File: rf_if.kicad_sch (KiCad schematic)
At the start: 46 parts, among them IC1 SBL-1+, Q33 2SC5171, U2 74LVC74, U3 Adafruit_Si5351, U4 74HCT244, U5 74HC4066, U6 74HC4066, U7 LM358

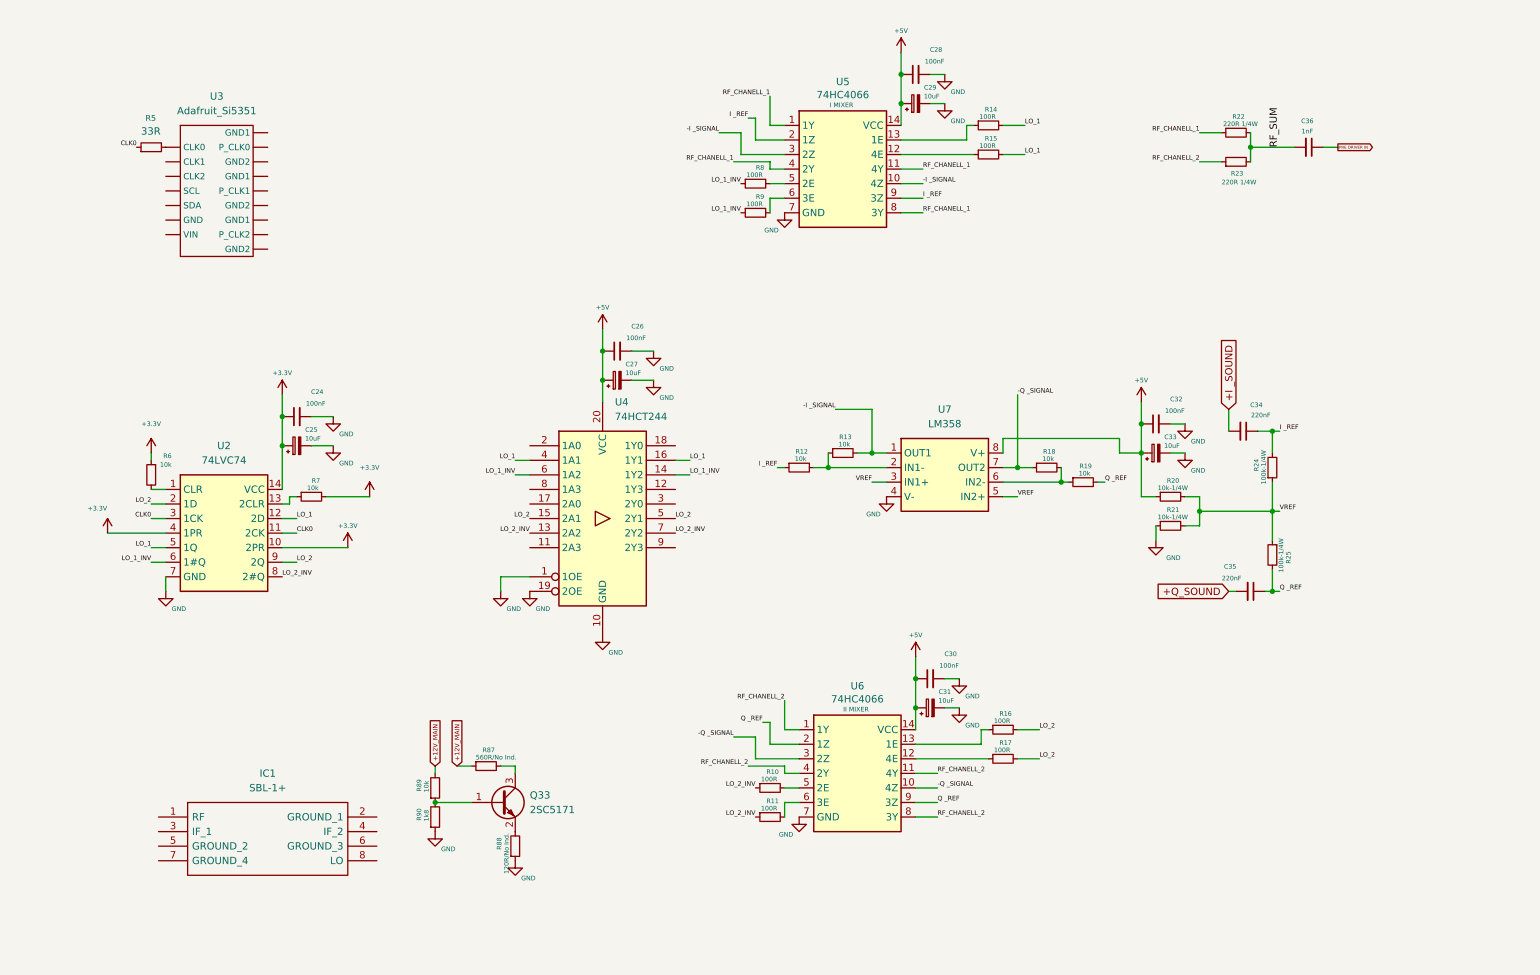
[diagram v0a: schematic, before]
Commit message: Mixer work 2
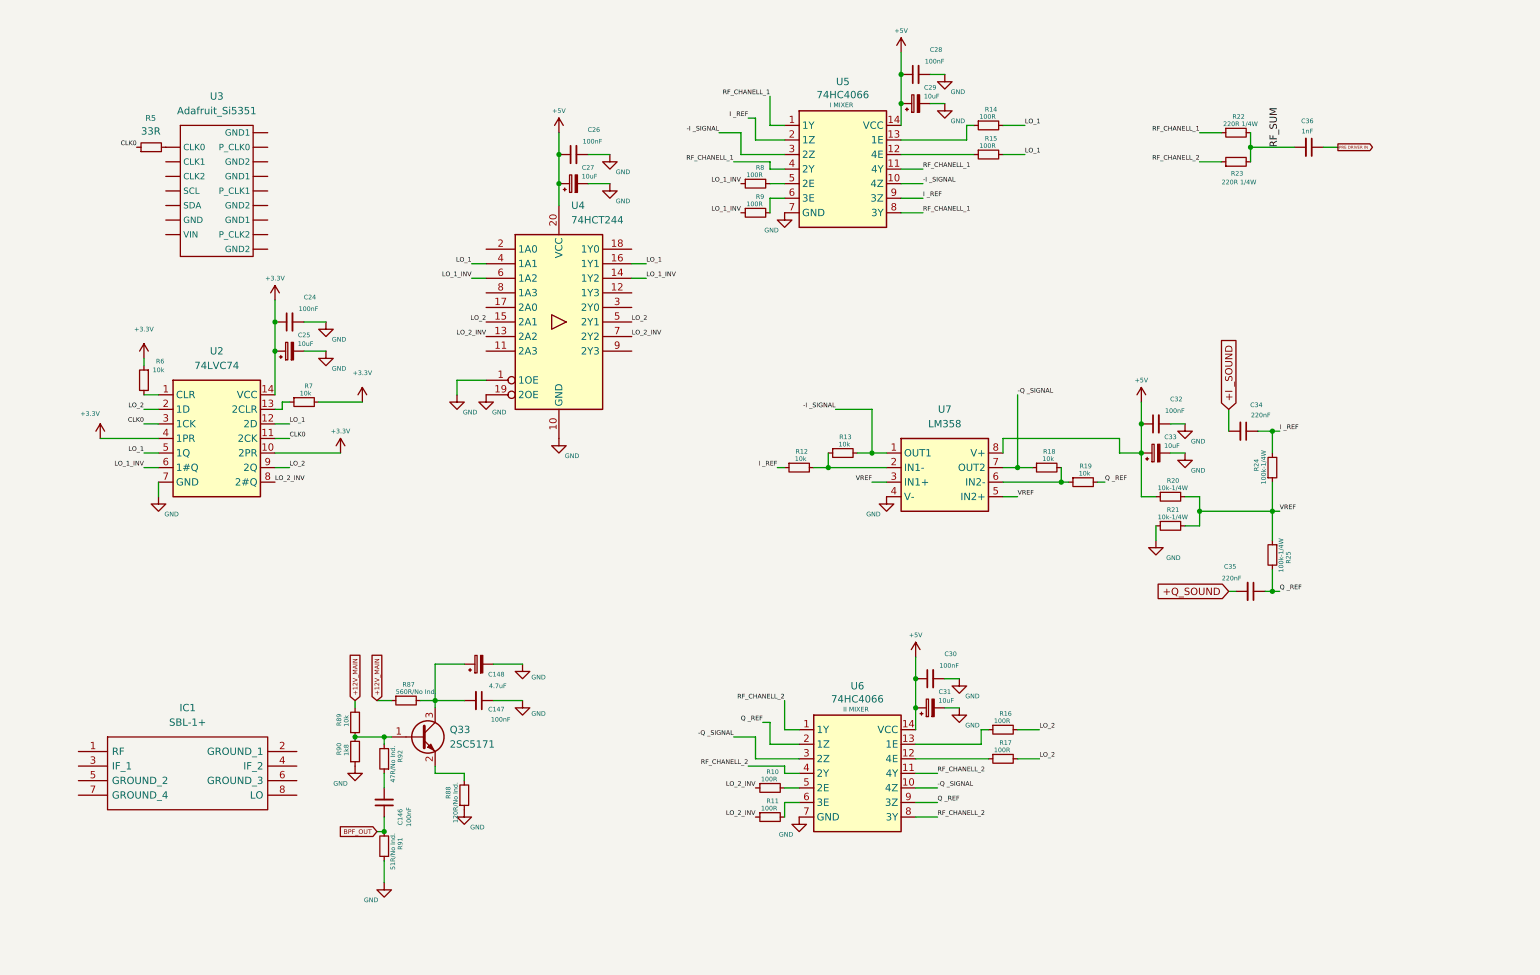
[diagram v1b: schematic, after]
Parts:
- added C146, C147: 100nF, symbol Device:C_Small
- added C148: 4.7uF, symbol Device:C_Polarized_Small
- added R91: 51R/No Ind., symbol Device:R_Small
- added R92: 47R/No Ind., symbol Device:R_Small
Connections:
- net GND: now also C147.1, C148.2, R91.1
- net at Q33.1 (B), R89.1, R90.2: now also R92.2
- net at Q33.3 (C), R87.2: now also C147.2, C148.1
- new net: C146.2, R92.1
- new net BPF_OUT: C146.1, R91.2
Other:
- moved on the sheet: C24, C25, C26, C27, IC1, Q33, R6, R7, R87, R88, R89, R90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

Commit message: Mixer work 3
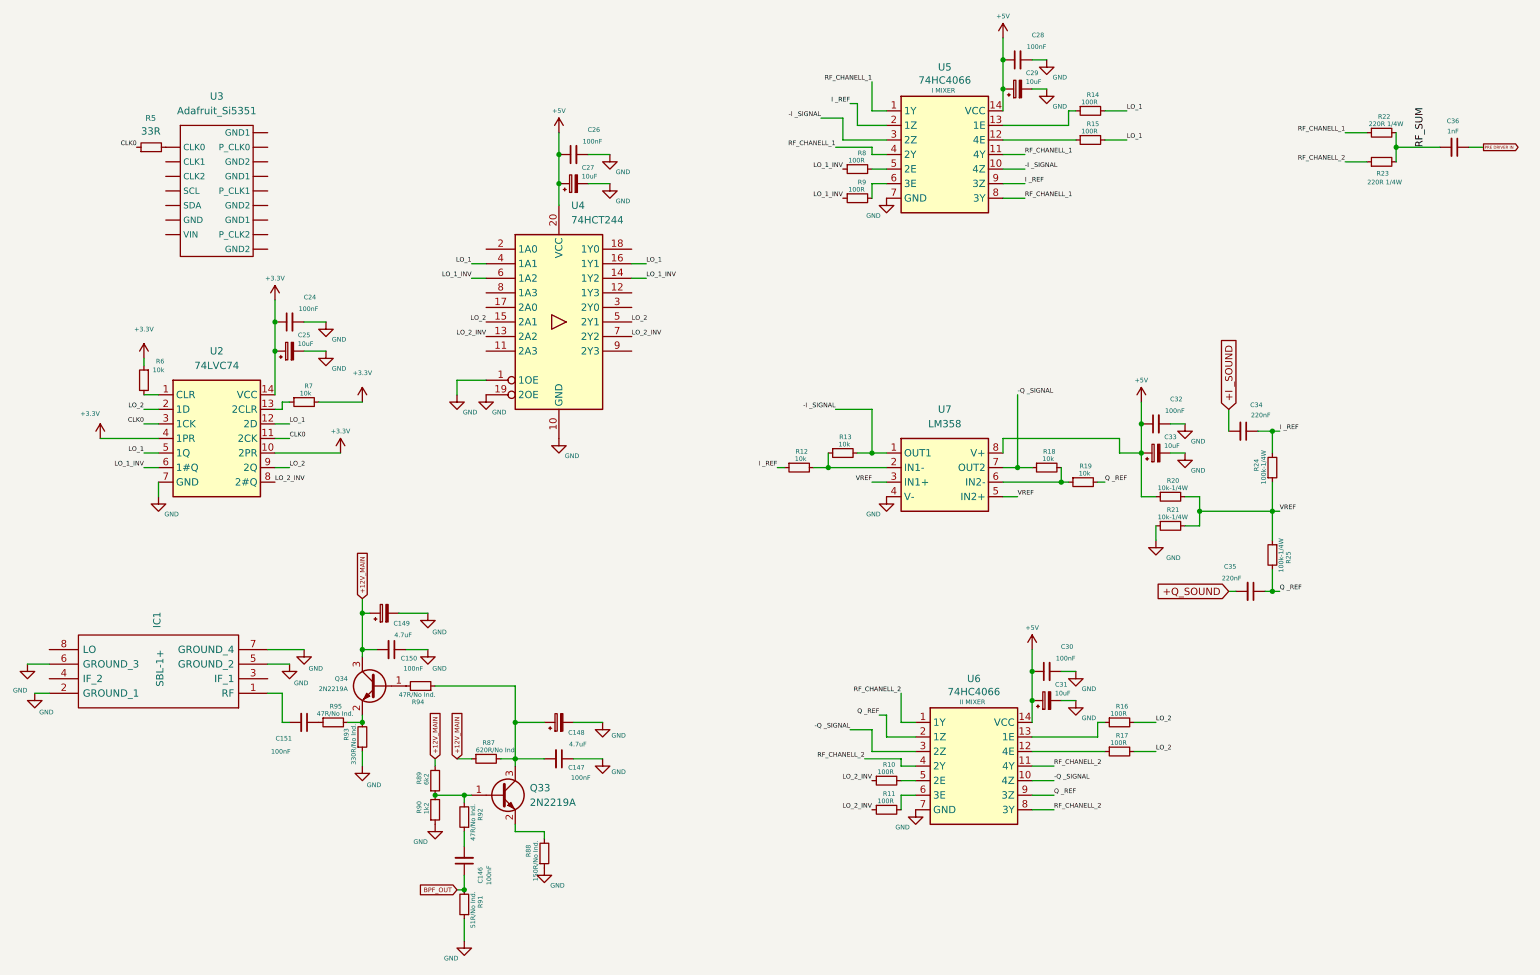
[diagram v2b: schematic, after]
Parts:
- added C149: 4.7uF, symbol Device:C_Polarized_Small
- added C150, C151: 100nF, symbol Device:C_Small
- added Q34: 2N2219A, Package_TO_SOT_THT:TO-220-3_Vertical, symbol Transistor_BJT:2SC1945
- added R93: 330R/No Ind., symbol Device:R_Small
- added R94, R95: 47R/No Ind., symbol Device:R_Small
- Q33: value 2SC5171 -> 2N2219A
- R87: value 560R/No Ind. -> 620R/No Ind.
- R88: value 120R/No Ind. -> 150R/No Ind.
- R89: value 10k -> 6k2
- R90: value 1k8 -> 1k2
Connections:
- net +12V_MAIN: now also C149.1, C150.2, Q34.3 (C)
- net GND: now also IC1.2 (GROUND_1), IC1.5 (GROUND_2), IC1.6 (GROUND_3), IC1.7 (GROUND_4), C149.2, C150.1, R93.1
- net at C147.2, C148.1, Q33.3 (C)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: now also R94.1
- net at IC1.1 (RF): now also C151.2
- new net: C151.1, R95.1
- new net: Q34.1 (B), R94.2
- new net: Q34.2 (E), R93.2, R95.2
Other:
- moved on the sheet: C146, C147, C148, C28, C29, C30, C31, C36, IC1, Q33, R10, R11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
